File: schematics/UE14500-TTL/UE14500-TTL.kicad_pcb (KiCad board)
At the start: 2 copper layers, 76.8 x 99.1 mm, 43 parts, among them J1 Edge 1, J2 Edge 2, J3 5VDC IN, SW1 Power On, U1 74LS08, U10 74LS74, U11 74LS00, U12 74LS86, U13 74LS00, U14 74LS151, U15 74LS02, U16 74LS74, U2 74LS08, U3 74LS00, U4 74LS374, U5 74LS138, U6 74LS138, U7 74LS74, U8 74LS02, U9 74LS02

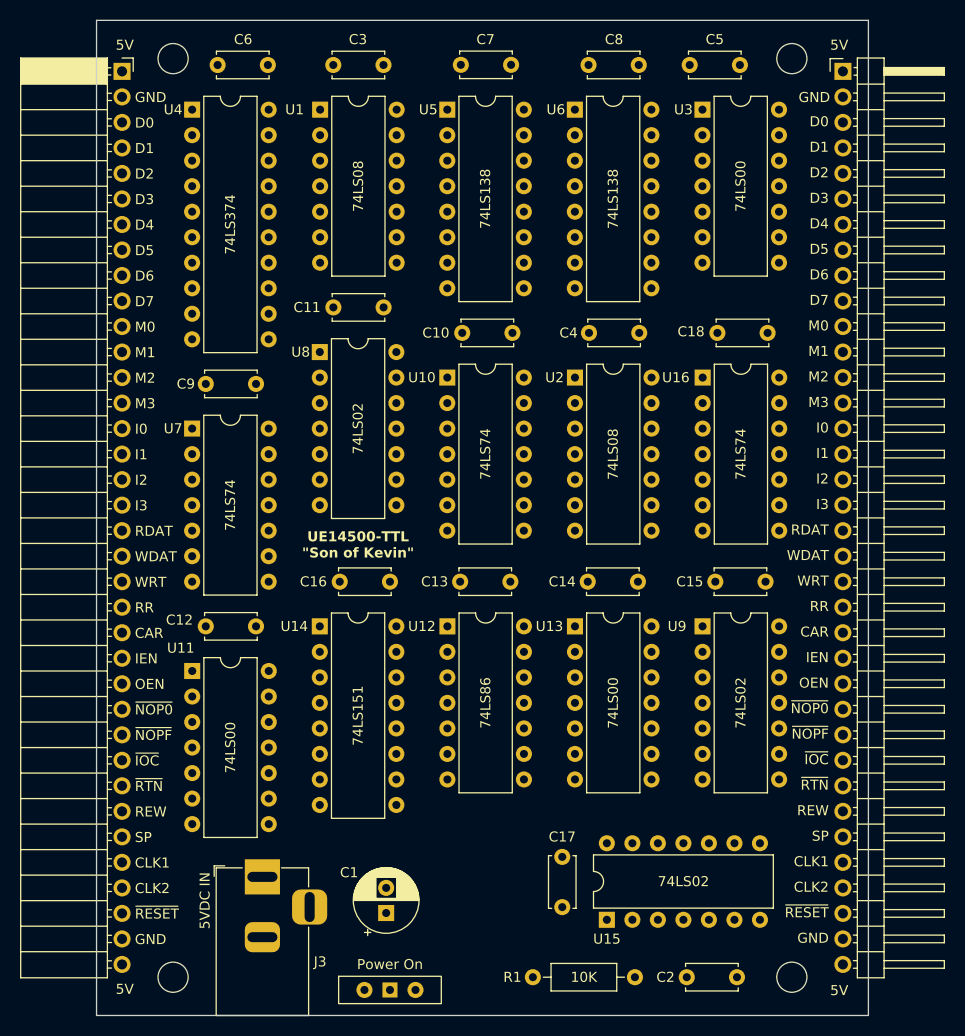
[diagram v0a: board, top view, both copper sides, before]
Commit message: Lay out CPU board
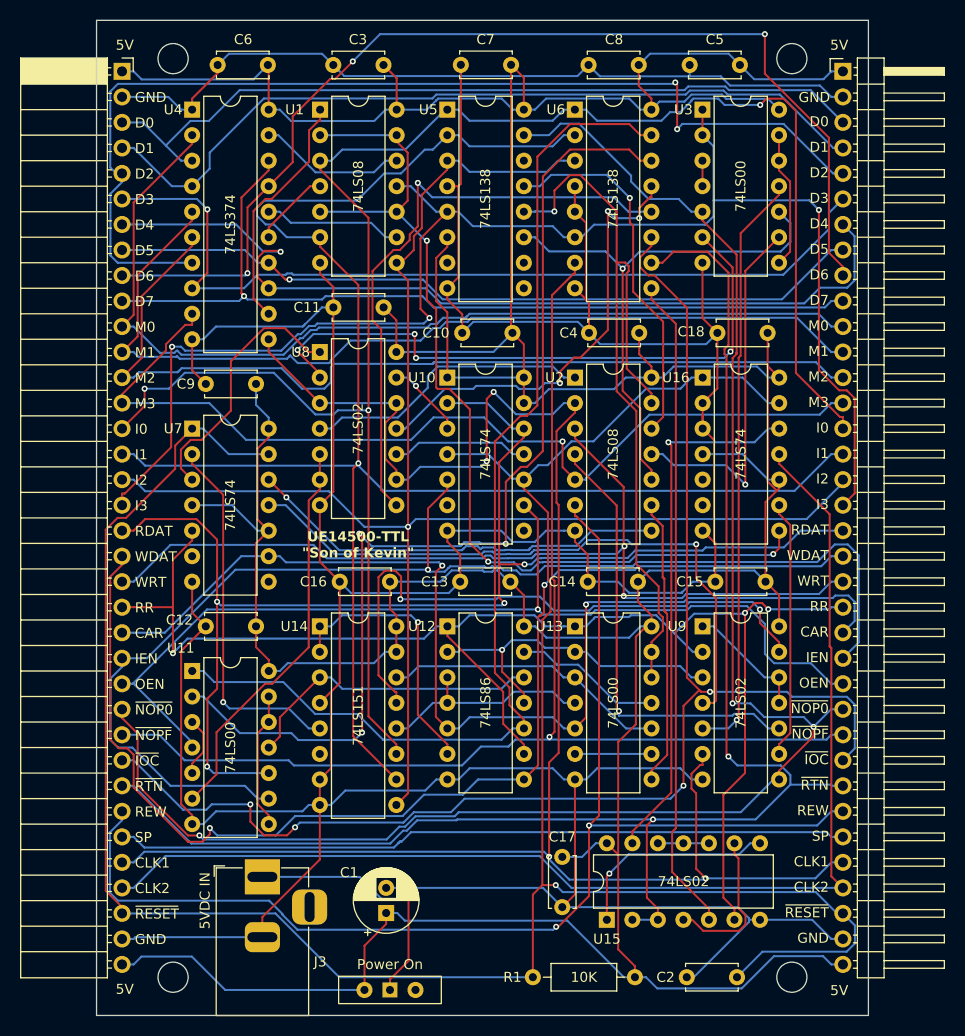
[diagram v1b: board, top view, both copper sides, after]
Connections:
- net CAR_VAL renamed CAR_ALU
- net RR_VAL renamed RR_ALU
- U16 pad 9: unconnected-(U16B-Q-Pad9) -> SKIP
- U2 pad 5: INST3 -> MEM3
- U9 pad 9: ~{OP_NOP0} -> SKIP
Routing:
- net +5V: track 0.00 -> 499.8 mm
- net GND: track 0.00 -> 499.7 mm
- net ~{RESET}: track 0.00 -> 244.4 mm, vias 0 -> 1
- net CLK1: track 0.00 -> 185.2 mm, vias 0 -> 4
- net INST0: track 0.00 -> 178.5 mm, vias 0 -> 3
- net INST1: track 0.00 -> 176.1 mm, vias 0 -> 1
- net ~{OP_NOP0}: track 0.00 -> 168.8 mm, vias 0 -> 3
- net INST2: track 0.00 -> 156.9 mm, vias 0 -> 1
- net ~{OP_RTN}: track 0.00 -> 155.2 mm, vias 0 -> 2
- net INST3: track 0.00 -> 145.5 mm, vias 0 -> 3
- net ~{OP_IOC}: track 0.00 -> 143.1 mm, vias 0 -> 4
- net RR: track 0.00 -> 140.9 mm, vias 0 -> 3
- net RD_DATA: track 0.00 -> 131.9 mm, vias 0 -> 4
- net IEN: track 0.00 -> 126.9 mm, vias 0 -> 1
- net REWIND: track 0.00 -> 125.5 mm, vias 0 -> 2
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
